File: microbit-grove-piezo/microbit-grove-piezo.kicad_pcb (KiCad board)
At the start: 2 copper layers, 59 x 15.4 mm, 8 parts, among them J1 microbit_smd_socket, J2 GROVE-CONNECTOR-SMD_4+2P-2.0_, J3 GROVE-CONNECTOR-SMD_4+2P-2.0_, J4 GROVE-CONNECTOR-SMD_4+2P-2.0_, J5 GROVE-CONNECTOR-SMD_4+2P-2.0_

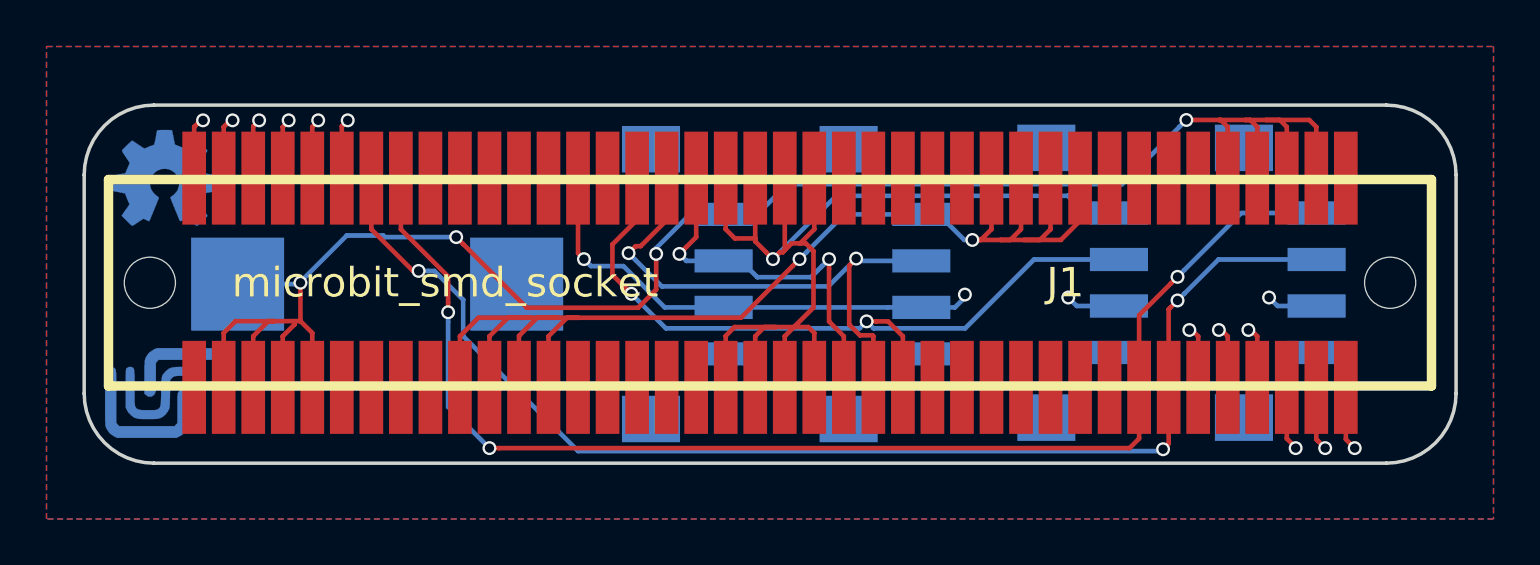
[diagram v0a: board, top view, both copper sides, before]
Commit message: Update fills.
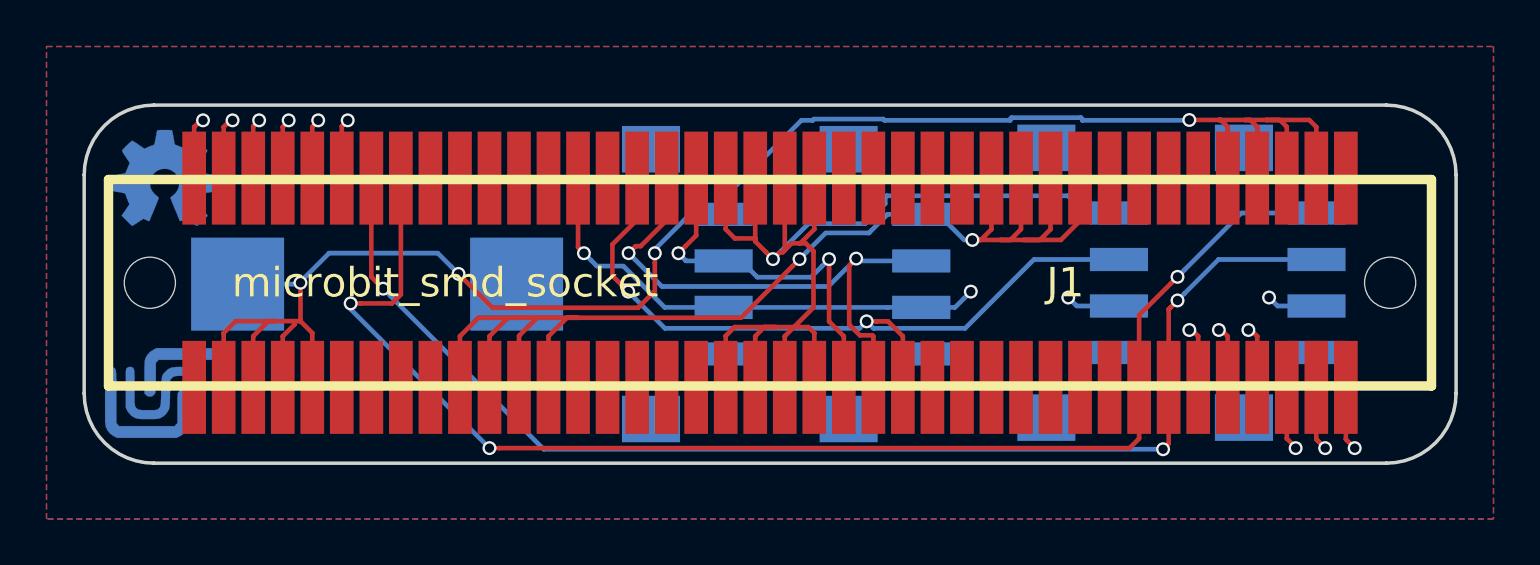
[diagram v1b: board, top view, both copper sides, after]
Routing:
- net MB_19: track 56.1 -> 58.9 mm
